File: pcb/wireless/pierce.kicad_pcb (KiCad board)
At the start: 2 copper layers, 112.2 x 91.4 mm, 27 parts, among them SW1 SW_PUSH, SW10 SW_PUSH, SW15 SW_PUSH, SW16 SW_PUSH, SW17 SW_PUSH, SW18 SW_PUSH, SW2 SW_PUSH, SW23 SW_PUSH, SW24 SW_PUSH, SW25 SW_PUSH, SW26 SW_PUSH, SW3 SW_PUSH, SW30 SW_PUSH, SW31 SW_PUSH, SW32 SW_PUSH, SW33 SW_PUSH, SW8 SW_PUSH, SW9 SW_PUSH

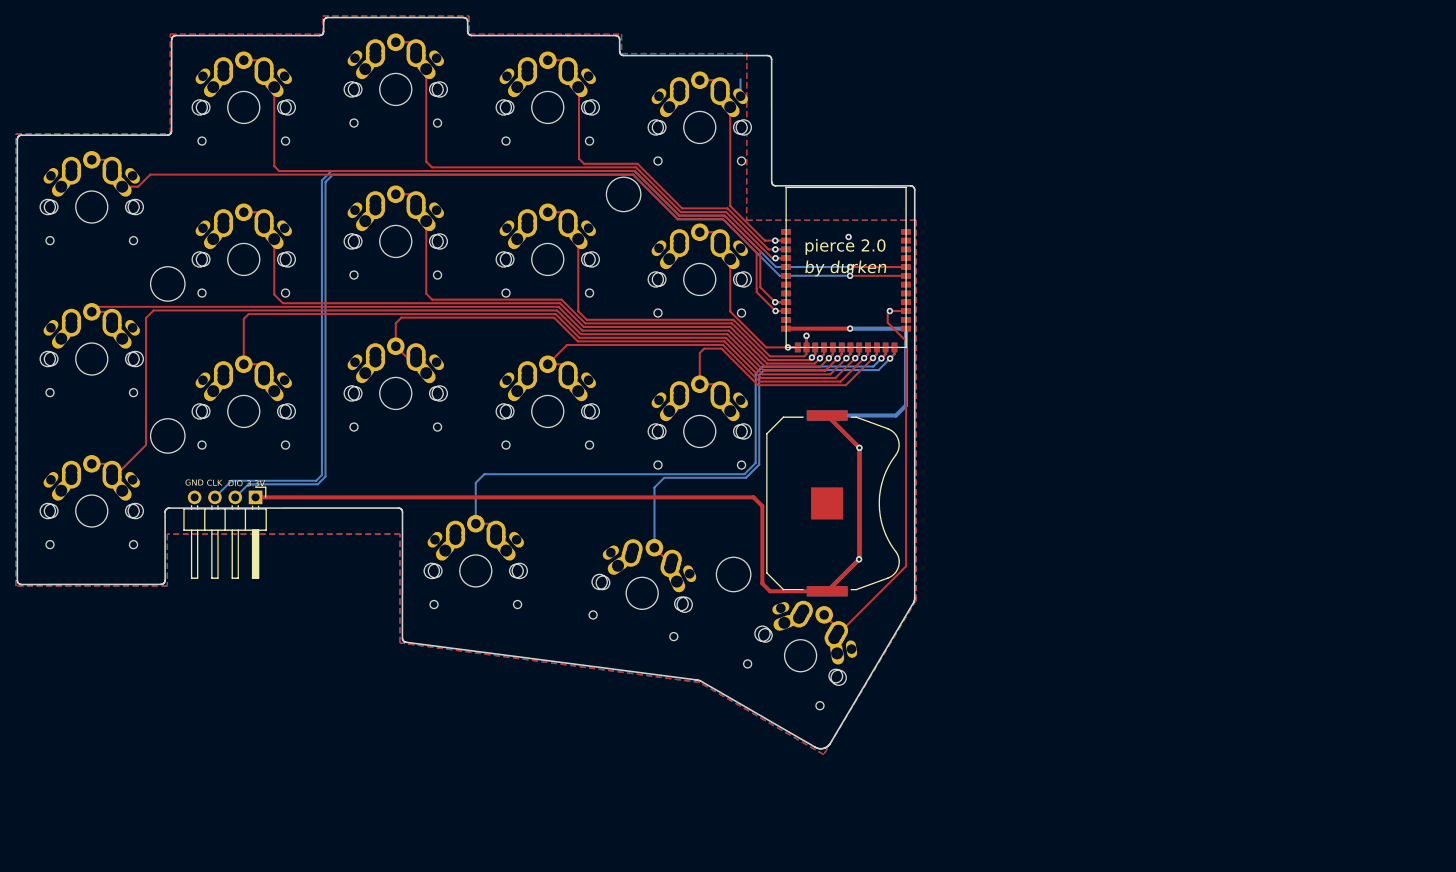
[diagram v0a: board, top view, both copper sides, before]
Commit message: prototype - ordered
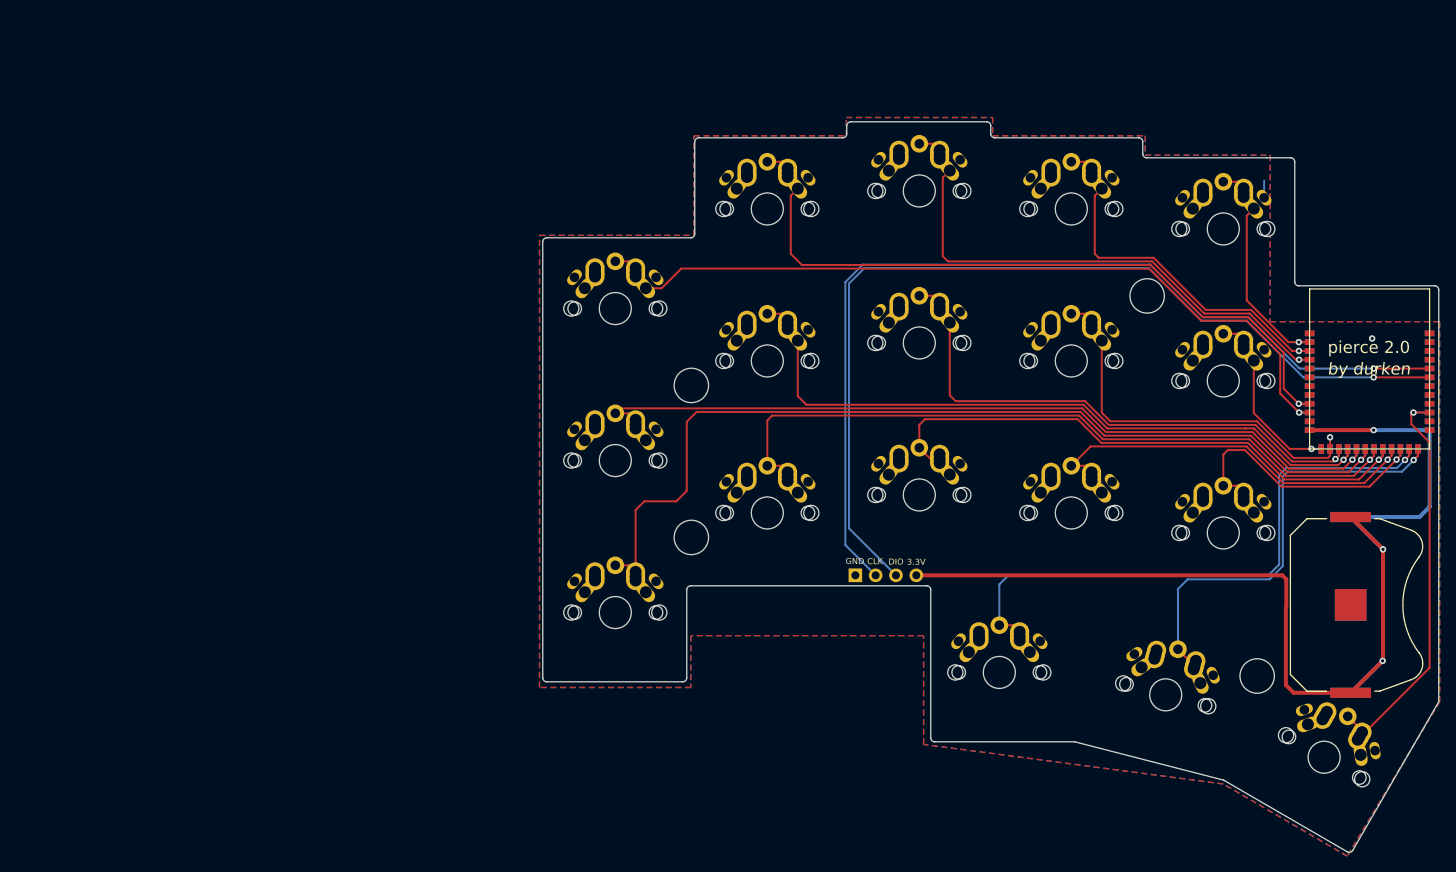
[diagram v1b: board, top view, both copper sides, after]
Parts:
- moved PROGL1 83.2 mm to (144.7, 93.7)
- moved SW26 66.7 mm to (175.9, 108.6)
- moved Ref** 66.7 mm to (173.6, 58.8)
- moved SW1 66.7 mm to (107.1, 60.3)
- moved SW30 66.7 mm to (183.1, 50.4)
- moved SW31 66.7 mm to (183.1, 69.4)
- moved SW32 66.7 mm to (183.1, 88.4)
- moved SW33 66.7 mm to (195.7, 116.4)
- moved SW2 66.7 mm to (107.1, 79.3)
- moved SW3 66.7 mm to (107.1, 98.3)
- moved BT1 66.7 mm to (199.0, 97.4)
- moved BT2 66.7 mm to (199.0, 97.4)
- moved Ref** 66.7 mm to (116.6, 89.0)
- moved Ref** 66.7 mm to (116.6, 70.0)
- moved SW10 66.7 mm to (126.1, 85.9)
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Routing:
- net VCC: track 167.6 -> 153.8 mm
- net CLKL: track 129.6 -> 117.3 mm
- net DIOL: track 127.2 -> 117.7 mm
- net SW03L: track 45.8 -> 46.6 mm
- net SW00L: track 99.7 -> 100.5 mm
- net SW02L: track 67.7 -> 68.5 mm
- net SW04L: track 27.4 -> 28.1 mm
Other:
- board size 112.2 x 91.4 mm -> 112 x 91.3 mm
- net class Default removed
